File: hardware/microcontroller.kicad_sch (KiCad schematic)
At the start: 5 parts, among them U1 ATSAMD21G18A-M

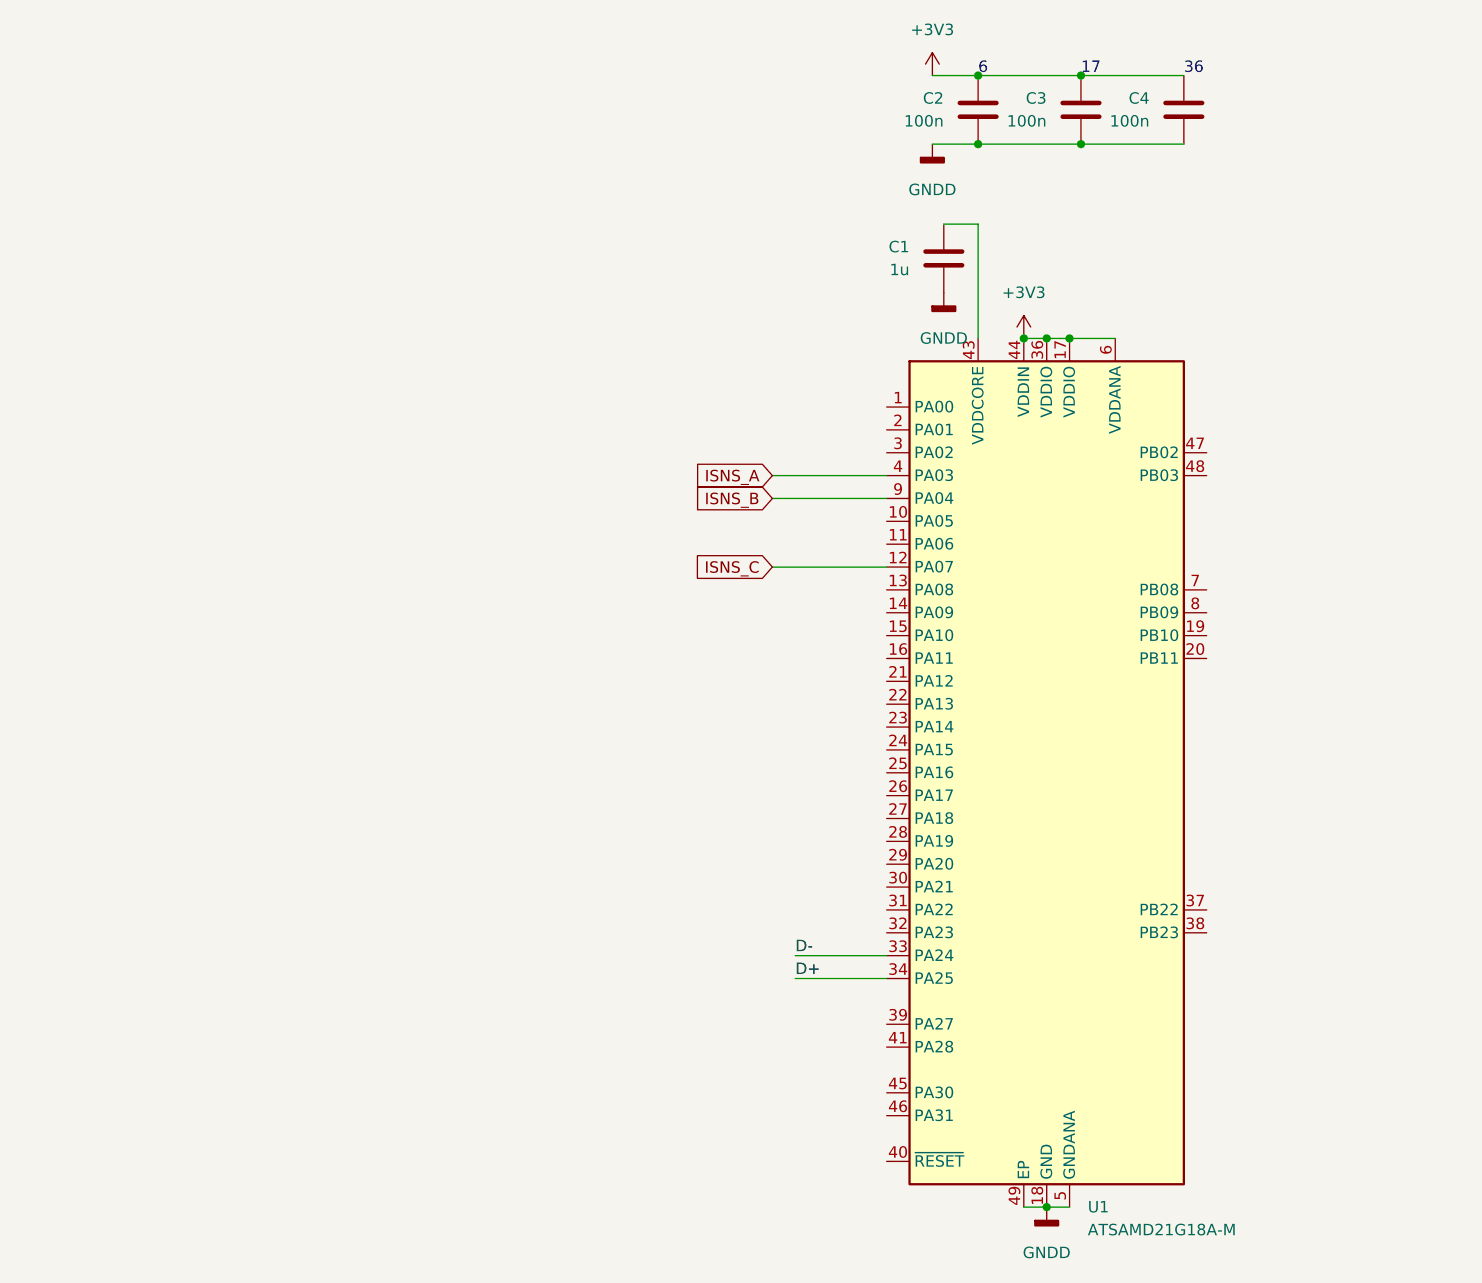
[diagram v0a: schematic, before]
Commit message: workin away
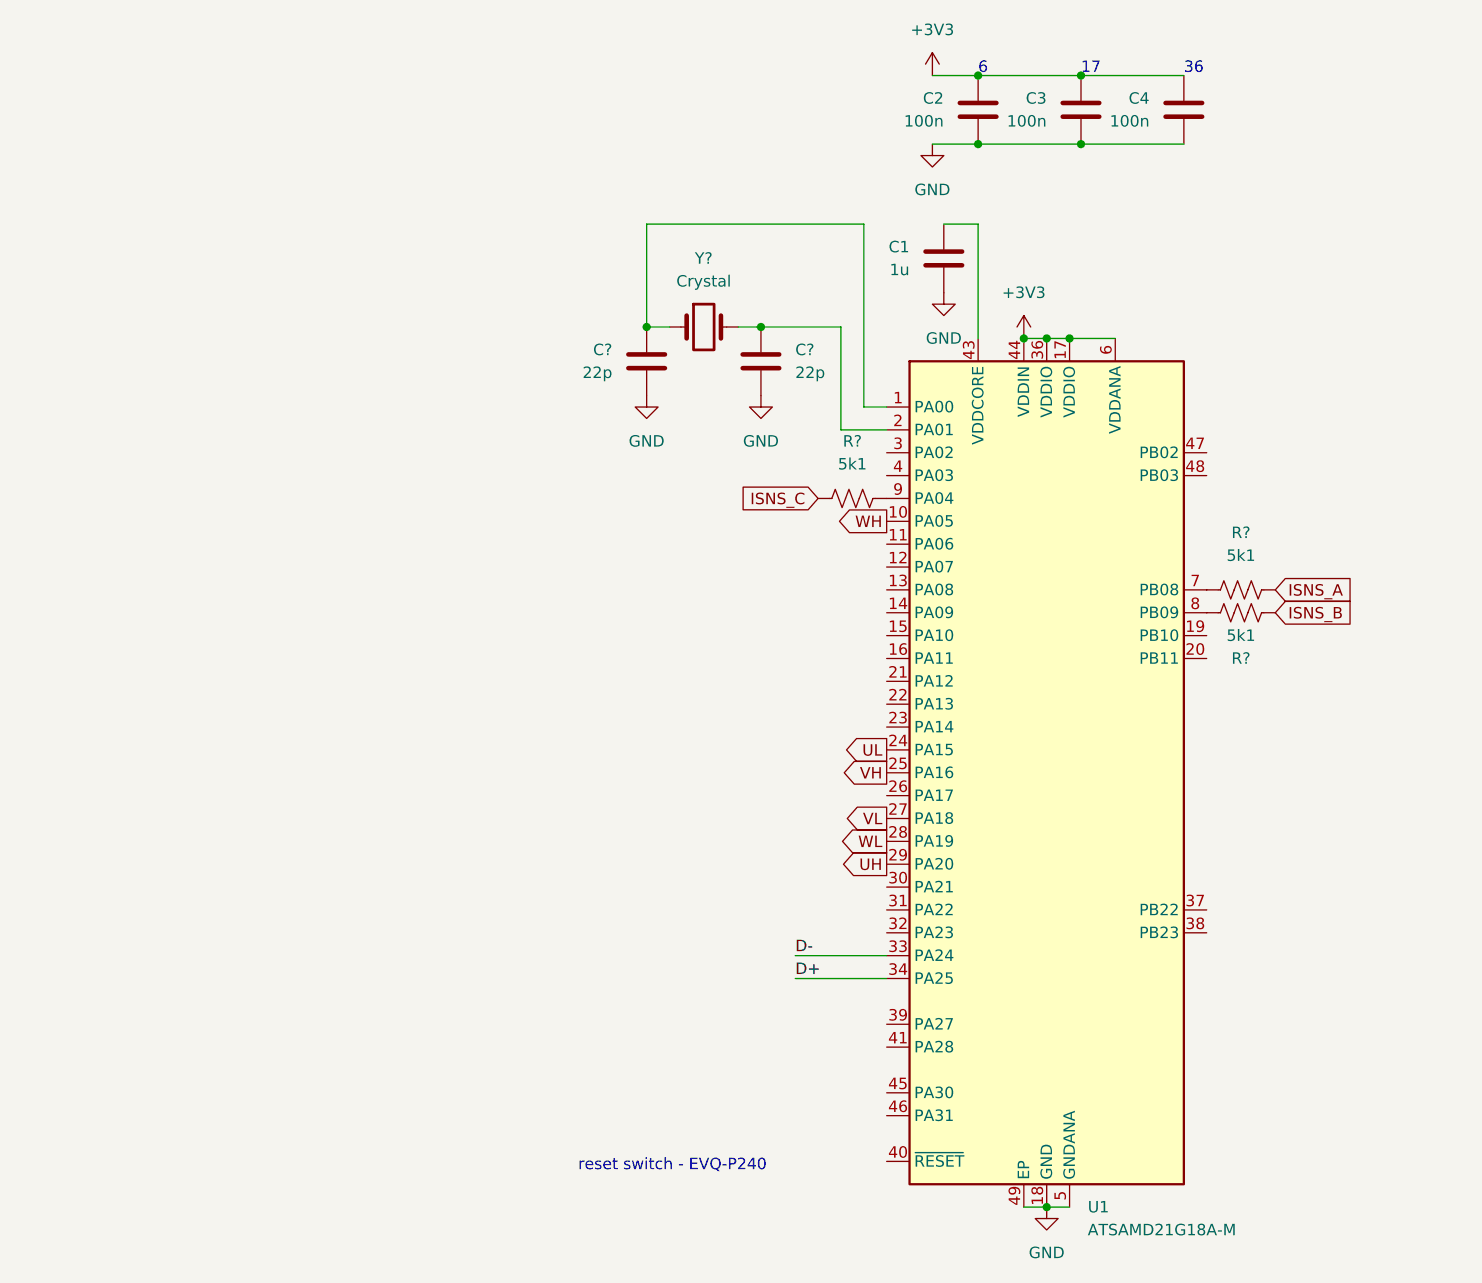
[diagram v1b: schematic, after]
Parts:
- added C? (x2): 22p, Capacitor_SMD:C_0402_1005Metric_Pad0.74x0.62mm_HandSolder, symbol Device:C
- added R? (x3): 5k1, Resistor_SMD:R_0805_2012Metric, symbol Device:R_US
- added Y?: Crystal, Crystal:Crystal_SMD_MicroCrystal_CC8V-T1A-2Pin_2.0x1.2mm, symbol Device:Crystal
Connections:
- net ISNS_A: now also R?.2; no longer U1.4 (PA03)
- net ISNS_B: now also R?.2; no longer U1.9 (PA04)
- net ISNS_C: now also R?.1; no longer U1.12 (PA07)
- net at U1.1 (PA00): now also C?.2, Y?.1
- net WH: now reaches U1.10 (PA05)
- net at U1.2 (PA01): now also C?.1, Y?.2
- net UL: now reaches U1.24 (PA15)
- net VH: now reaches U1.25 (PA16)
- net VL: now reaches U1.27 (PA18)
- net WL: now reaches U1.28 (PA19)
- net UH: now reaches U1.29 (PA20)
- net at U1.7 (PB08): now also R?.1
- net at U1.8 (PB09): now also R?.1
- net GNDD renamed GND
- net GND: now also C?.1, C?.2
- new net: R?.2, U1.9 (PA04)
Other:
- note added: "reset switch - EVQ-P240"

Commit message: microcontroller done?
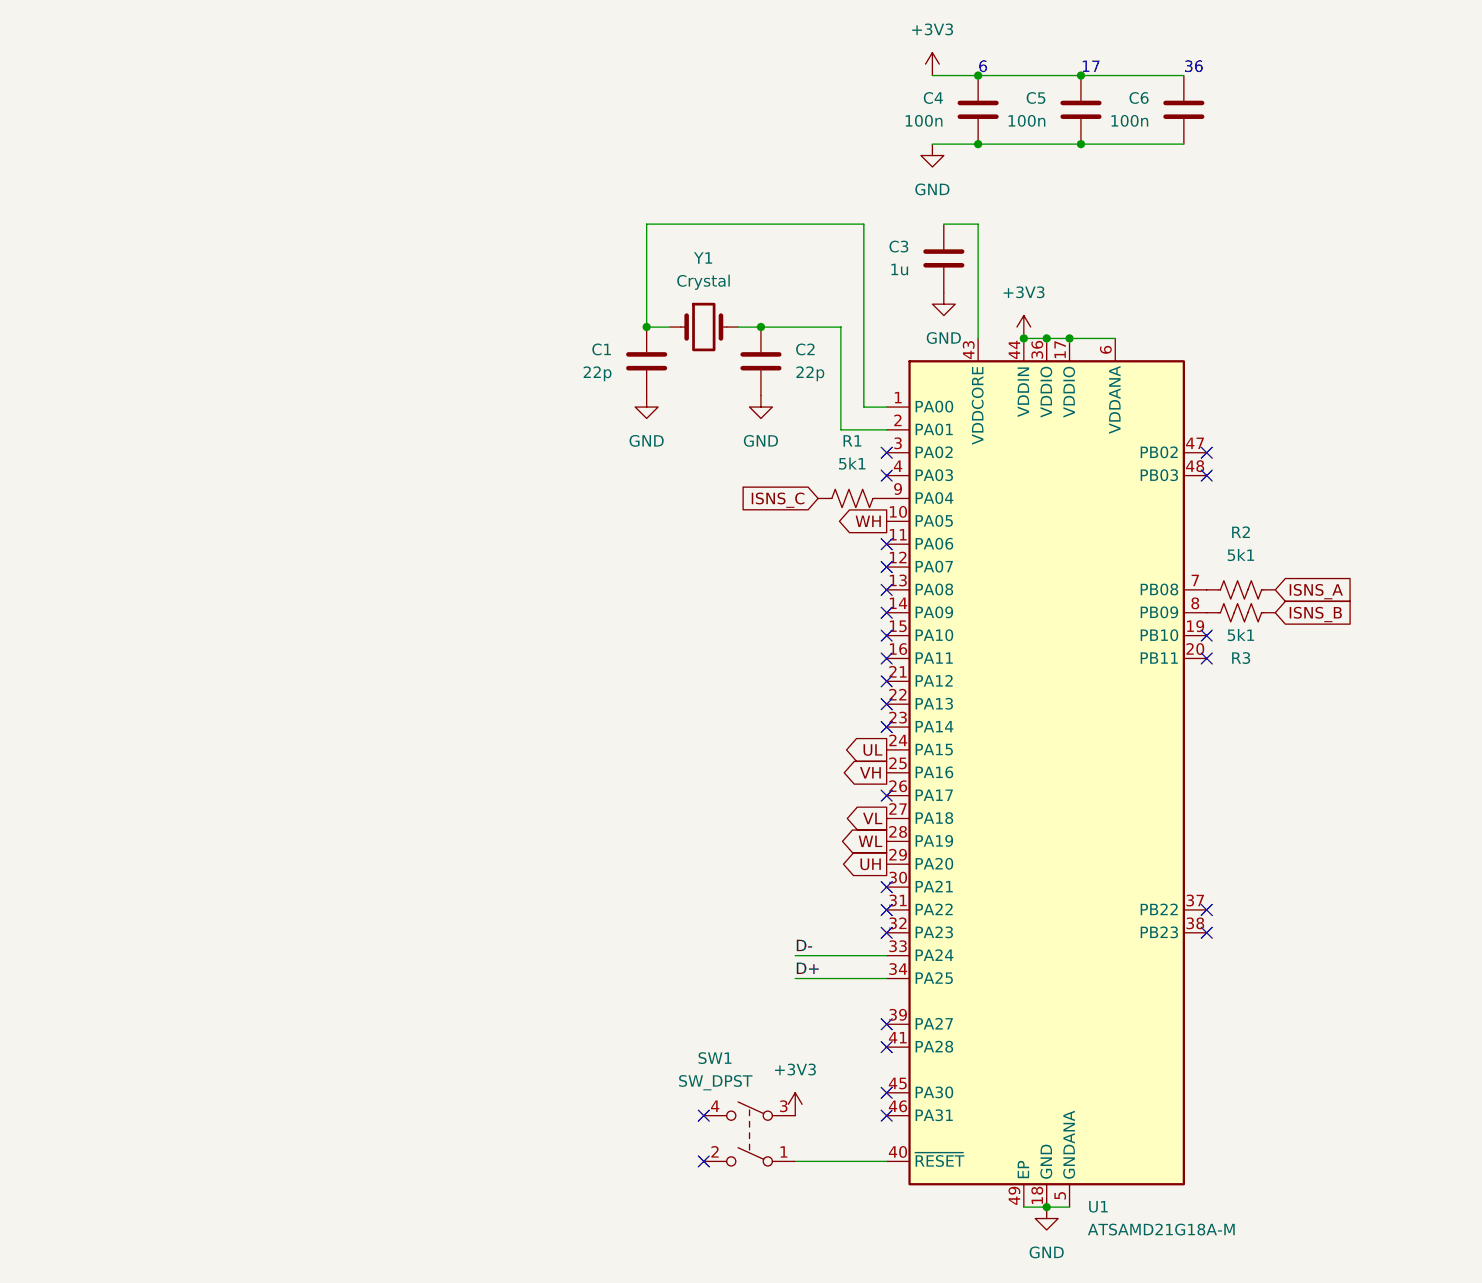
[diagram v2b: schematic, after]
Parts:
- added SW1: SW_DPST, EVQ-P2402M:EVQ-P2402M, symbol Switch:SW_DPST
- gave numbers to parts that had none: 6
- renumbered C1 to C3, C2 to C4, C3 to C5, C4 to C6
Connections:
- net +3V3: now also SW1.3
- net at U1.40 (~{RESET}): now also SW1.1
- no-connect marks 0 -> 27
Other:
- note removed: "reset switch - EVQ-P240"
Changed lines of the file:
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@@
   (junction (at 95.25 52.07) (diameter 0) (color 0 0 0 0)
   )
+  (no_connect (at 121.92 66.04))
+  (no_connect (at 121.92 68.58))
+  (no_connect (at 121.92 76.2))
+  (no_connect (at 121.92 78.74))
+  (no_connect (at 121.92 81.28))
+  (no_connect (at 121.92 96.52))
+  (no_connect (at 157.48 116.84))
+  (no_connect (at 157.48 119.38))
+  (no_connect (at 157.48 88.9))
+  (no_connect (at 157.48 86.36))
+  (no_connect (at 121.92 83.82))
+  (no_connect (at 121.92 86.36))
+  (no_connect (at 121.92 88.9))
+  (no_connect (at 121.92 91.44))
+  (no_connect (at 121.92 93.98))
+  (no_connect (at 157.48 66.04))
+  (no_connect (at 157.48 68.58))
+  (no_connect (at 101.6 139.7))
+  (no_connect (at 101.6 144.78))
+  (no_connect (at 121.92 119.38))
+  (no_connect (at 121.92 116.84))
+  (no_connect (at 121.92 114.3))
+  (no_connect (at 121.92 104.14))
+  (no_connect (at 121.92 139.7))
+  (no_connect (at 121.92 137.16))
+  (no_connect (at 121.92 132.08))
+  (no_connect (at 121.92 129.54))
   (wire (pts (xy 132.08 31.75) (xy 143.51 31.75))
     (stroke (width 0) (type default) (color 0 0 0 0))
@@
   )
   (wire (pts (xy 137.16 53.34) (xy 139.7 53.34))
+    (stroke (width 0) (type default) (color 0 0 0 0))
+  )
+  (wire (pts (xy 111.76 144.78) (xy 121.92 144.78))
     (stroke (width 0) (type default) (color 0 0 0 0))
   )
@@
   )
   (text "36" (at 154.94 24.13 0)
-    (effects (font (size 1.27 1.27)) (justify left bottom))
-  )
-  (text "reset switch - EVQ-P240" (at 87.63 146.05 0)
     (effects (font (size 1.27 1.27)) (justify left bottom))
   )
@@
   (symbol (lib_id "power:+3V3") (at 127 24.13 0) (unit 1)
     (in_bom yes) (on_board yes) (fields_autoplaced)
-    (property "Reference" "#PWR01" (id 0) (at 127 27.94 0)
+    (property "Reference" "#PWR04" (id 0) (at 127 27.94 0)
       (effects (font (size 1.27 1.27)) hide)
     )
@@
     (pin "1")
   )
+  (symbol (lib_id "Switch:SW_DPST") (at 106.68 142.24 0) (mirror y) (unit 1)
+    (in_bom yes) (on_board yes)
+    (property "Reference" "SW1" (id 0) (at 102.87 133.35 0))
+    (property "Value" "SW_DPST" (id 1) (at 102.87 135.89 0))
+    (property "Footprint" "EVQ-P2402M:EVQ-P2402M" (id 2) (at 106.68 142.24 0)
+      (effects (font (size 1.27 1.27)) hide)
+    )
+    (property "Datasheet" "~" (id 3) (at 106.68 142.24 0)
+      (effects (font (size 1.27 1.27)) hide)
+    )
+    (property "Mouser" "https://www.mouser.com/ProductDetail/Panasonic/EVQ-P2402M?qs=SxaZfIVsCL0Vzf2d76%252BKCA%3D%3D" (id 4) (at 106.68 142.24 0)
+      (effects (font (size 1.27 1.27)) hide)
+    )
+    (pin "1")
+    (pin "2")
+    (pin "3")
+    (pin "4")
+  )
   (symbol (lib_id "power:GND") (at 127 31.75 0) (unit 1)
     (in_bom yes) (on_board yes) (fields_autoplaced)
-    (property "Reference" "#PWR?" (id 0) (at 127 38.1 0)
+    (property "Reference" "#PWR05" (id 0) (at 127 38.1 0)
       (effects (font (size 1.27 1.27)) hide)
     )
@@
   (symbol (lib_id "Device:C") (at 95.25 55.88 0) (mirror x) (unit 1)
     (in_bom yes) (on_board yes) (fields_autoplaced)
-    (property "Reference" "C?" (id 0) (at 91.44 54.6099 0)
+    (property "Reference" "C1" (id 0) (at 91.44 54.6099 0)
       (effects (font (size 1.27 1.27)) (justify right))
     )
@@
   (symbol (lib_id "Device:Crystal") (at 101.6 52.07 0) (unit 1)
     (in_bom yes) (on_board yes) (fields_autoplaced)
-    (property "Reference" "Y?" (id 0) (at 101.6 44.45 0))
+    (property "Reference" "Y1" (id 0) (at 101.6 44.45 0))
     (property "Value" "Crystal" (id 1) (at 101.6 46.99 0))
     (property "Footprint" "Crystal:Crystal_SMD_MicroCrystal_CC8V-T1A-2Pin_2.0x1.2mm" (id 2) (at 101.6 52.07 0)
@@
   (symbol (lib_id "power:GND") (at 107.95 59.69 0) (unit 1)
     (in_bom yes) (on_board yes) (fields_autoplaced)
-    (property "Reference" "#PWR?" (id 0) (at 107.95 66.04 0)
+    (property "Reference" "#PWR02" (id 0) (at 107.95 66.04 0)
       (effects (font (size 1.27 1.27)) hide)
     )
@@
   (symbol (lib_id "Device:C") (at 132.08 27.94 0) (mirror x) (unit 1)
     (in_bom yes) (on_board yes) (fields_autoplaced)
-    (property "Reference" "C2" (id 0) (at 128.27 26.6699 0)
+    (property "Reference" "C4" (id 0) (at 128.27 26.6699 0)
       (effects (font (size 1.27 1.27)) (justify right))
     )
@@
   (symbol (lib_id "power:GND") (at 128.27 48.26 0) (unit 1)
     (in_bom yes) (on_board yes) (fields_autoplaced)
-    (property "Reference" "#PWR?" (id 0) (at 128.27 54.61 0)
+    (property "Reference" "#PWR06" (id 0) (at 128.27 54.61 0)
       (effects (font (size 1.27 1.27)) hide)
     )
@@
   (symbol (lib_id "Device:C") (at 143.51 27.94 0) (mirror x) (unit 1)
     (in_bom yes) (on_board yes) (fields_autoplaced)
-    (property "Reference" "C3" (id 0) (at 139.7 26.6699 0)
+    (property "Reference" "C5" (id 0) (at 139.7 26.6699 0)
       (effects (font (size 1.27 1.27)) (justify right))
     )
@@
   (symbol (lib_id "Device:C") (at 128.27 44.45 0) (mirror x) (unit 1)
     (in_bom yes) (on_board yes) (fields_autoplaced)
-    (property "Reference" "C1" (id 0) (at 124.46 43.1799 0)
+    (property "Reference" "C3" (id 0) (at 124.46 43.1799 0)
       (effects (font (size 1.27 1.27)) (justify right))
     )
@@
   (symbol (lib_id "Device:R_US") (at 161.29 83.82 90) (unit 1)
     (in_bom yes) (on_board yes)
-    (property "Reference" "R?" (id 0) (at 161.29 88.9 90))
+    (property "Reference" "R3" (id 0) (at 161.29 88.9 90))
     (property "Value" "5k1" (id 1) (at 161.29 86.36 90))
     (property "Footprint" "Resistor_SMD:R_0805_2012Metric" (id 2) (at 161.544 82.804 90)
@@
   (symbol (lib_id "power:GND") (at 95.25 59.69 0) (unit 1)
     (in_bom yes) (on_board yes) (fields_autoplaced)
-    (property "Reference" "#PWR?" (id 0) (at 95.25 66.04 0)
+    (property "Reference" "#PWR01" (id 0) (at 95.25 66.04 0)
       (effects (font (size 1.27 1.27)) hide)
     )
@@
   (symbol (lib_id "power:+3V3") (at 137.16 53.34 0) (unit 1)
     (in_bom yes) (on_board yes) (fields_autoplaced)
-    (property "Reference" "#PWR04" (id 0) (at 137.16 57.15 0)
+    (property "Reference" "#PWR07" (id 0) (at 137.16 57.15 0)
       (effects (font (size 1.27 1.27)) hide)
     )
@@
   (symbol (lib_id "power:GND") (at 139.7 149.86 0) (unit 1)
     (in_bom yes) (on_board yes) (fields_autoplaced)
-    (property "Reference" "#PWR?" (id 0) (at 139.7 156.21 0)
+    (property "Reference" "#PWR08" (id 0) (at 139.7 156.21 0)
       (effects (font (size 1.27 1.27)) hide)
     )
@@
   (symbol (lib_id "Device:R_US") (at 118.11 71.12 90) (unit 1)
     (in_bom yes) (on_board yes) (fields_autoplaced)
-    (property "Reference" "R?" (id 0) (at 118.11 64.77 90))
+    (property "Reference" "R1" (id 0) (at 118.11 64.77 90))
     (property "Value" "5k1" (id 1) (at 118.11 67.31 90))
     (property "Footprint" "Resistor_SMD:R_0805_2012Metric" (id 2) (at 118.364 70.104 90)
@@
   (symbol (lib_id "Device:R_US") (at 161.29 81.28 90) (unit 1)
     (in_bom yes) (on_board yes) (fields_autoplaced)
-    (property "Reference" "R?" (id 0) (at 161.29 74.93 90))
+    (property "Reference" "R2" (id 0) (at 161.29 74.93 90))
     (property "Value" "5k1" (id 1) (at 161.29 77.47 90))
     (property "Footprint" "Resistor_SMD:R_0805_2012Metric" (id 2) (at 161.544 80.264 90)
@@
   (symbol (lib_id "Device:C") (at 154.94 27.94 0) (mirror x) (unit 1)
     (in_bom yes) (on_board yes) (fields_autoplaced)
-    (property "Reference" "C4" (id 0) (at 151.13 26.6699 0)
+    (property "Reference" "C6" (id 0) (at 151.13 26.6699 0)
       (effects (font (size 1.27 1.27)) (justify right))
     )
@@
   (symbol (lib_id "Device:C") (at 107.95 55.88 0) (unit 1)
     (in_bom yes) (on_board yes) (fields_autoplaced)
-    (property "Reference" "C?" (id 0) (at 111.76 54.6099 0)
+    (property "Reference" "C2" (id 0) (at 111.76 54.6099 0)
       (effects (font (size 1.27 1.27)) (justify left))
     )
@@
     (pin "2")
   )
+  (symbol (lib_id "power:+3V3") (at 111.76 139.7 0) (unit 1)
+    (in_bom yes) (on_board yes) (fields_autoplaced)
+    (property "Reference" "#PWR03" (id 0) (at 111.76 143.51 0)
+      (effects (font (size 1.27 1.27)) hide)
+    )
+    (property "Value" "+3V3" (id 1) (at 111.76 134.62 0))
+    (property "Footprint" "" (id 2) (at 111.76 139.7 0)
+      (effects (font (size 1.27 1.27)) hide)
+    )
+    (property "Datasheet" "" (id 3) (at 111.76 139.7 0)
+      (effects (font (size 1.27 1.27)) hide)
+    )
+    (pin "1")
+  )
   (symbol (lib_id "MCU_Microchip_SAMD:ATSAMD21G18A-M") (at 139.7 101.6 0) (unit 1)
